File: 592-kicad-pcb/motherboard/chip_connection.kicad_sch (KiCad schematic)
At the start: 28 parts, among them J3 DF40C-40DP-0.4V(51), J4 DF40C-40DP-0.4V(51), J5 Conn_01x16, J6 Conn_01x16, J7 Conn_01x16

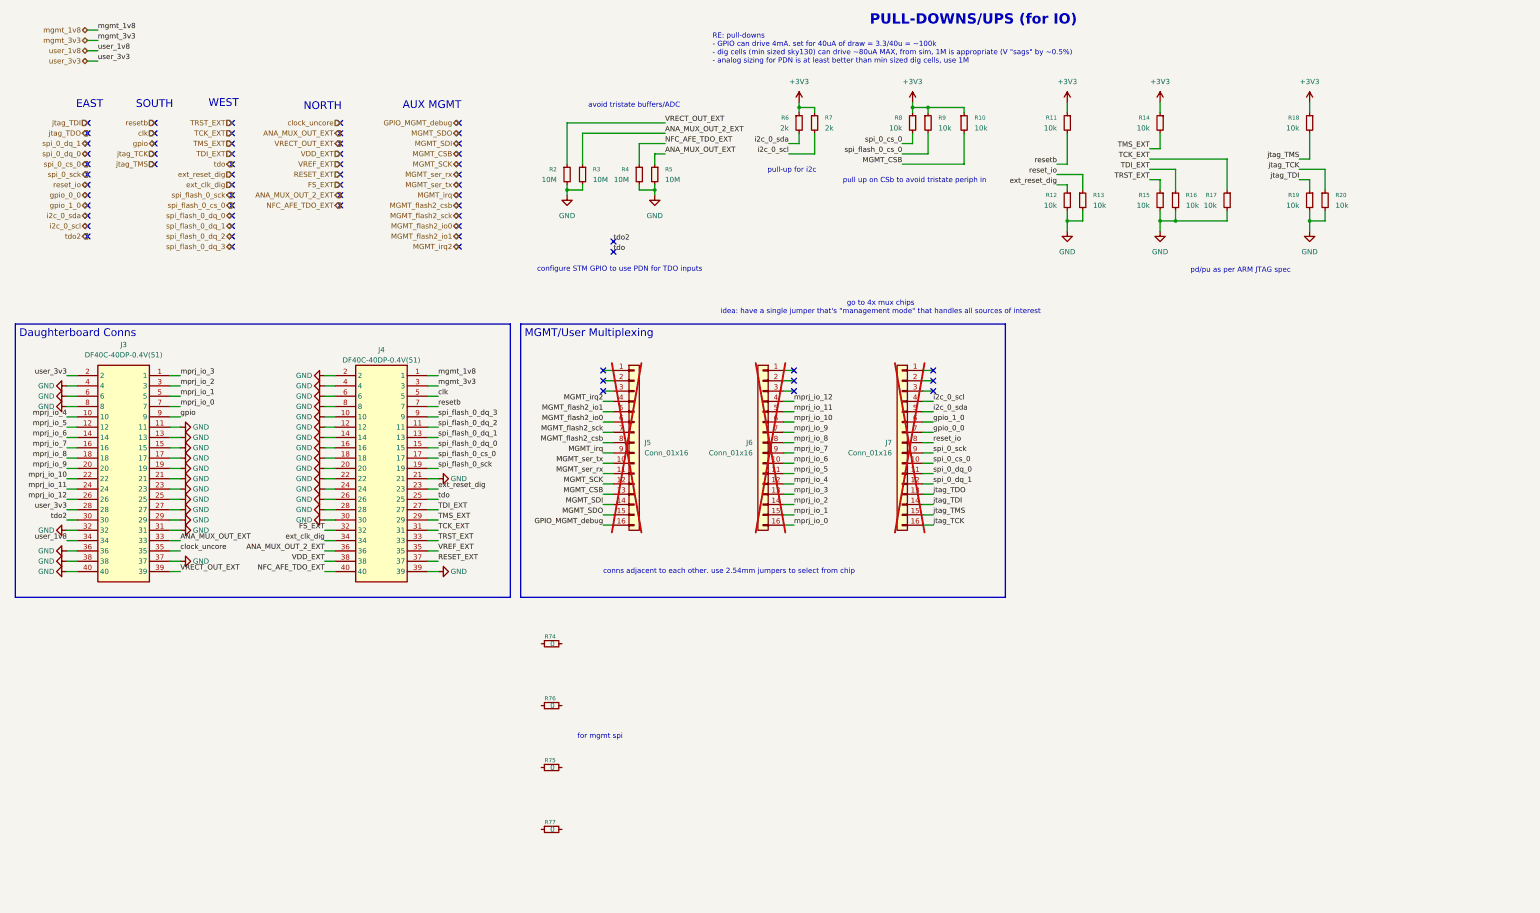
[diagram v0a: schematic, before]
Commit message: finalize termination
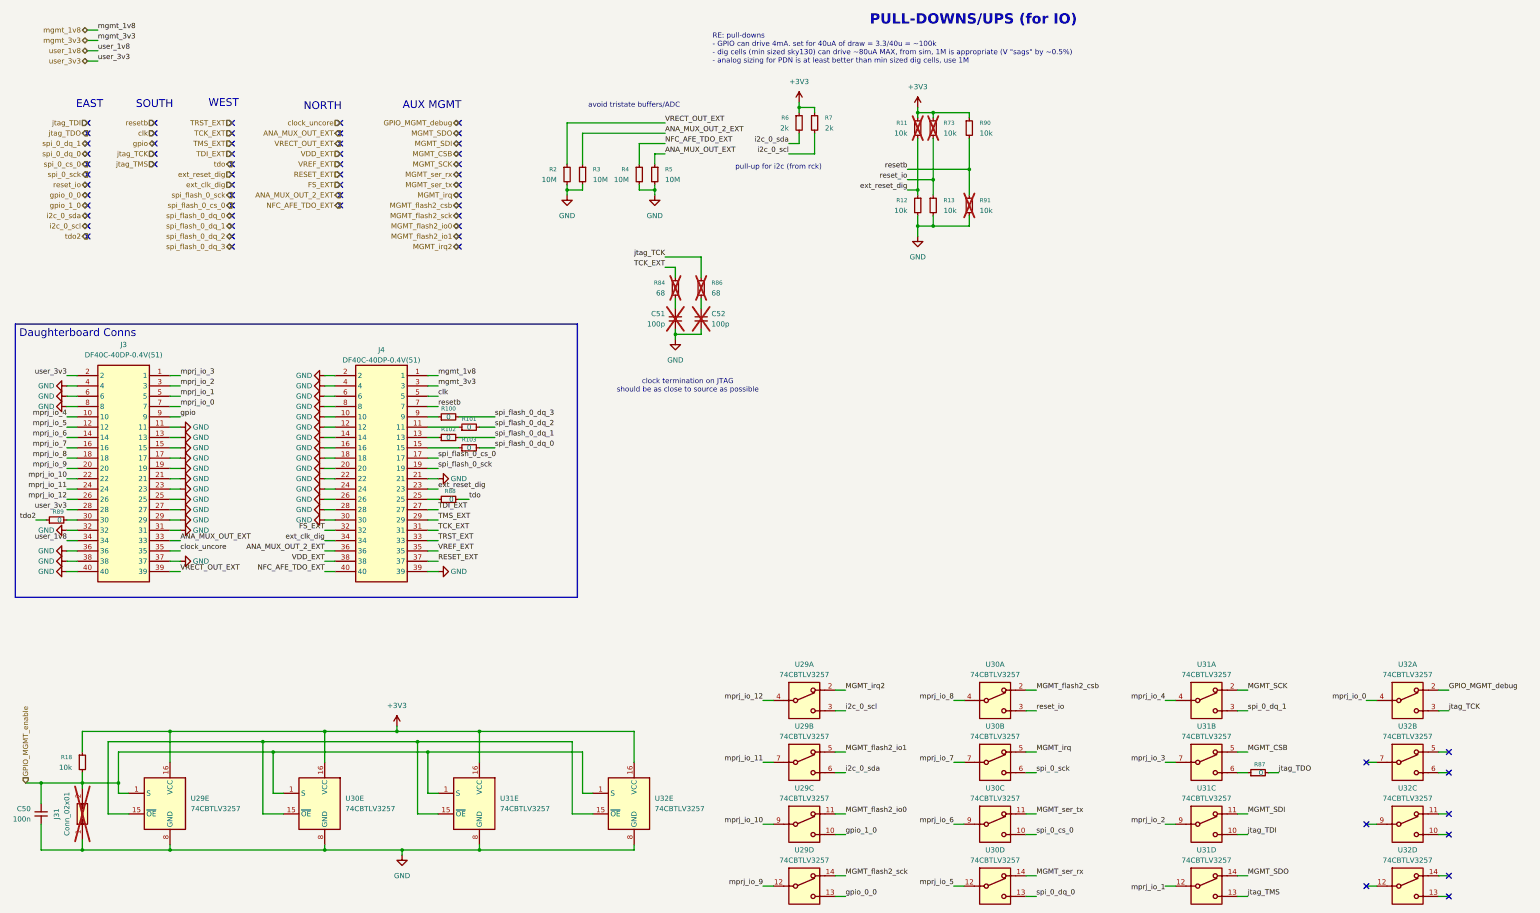
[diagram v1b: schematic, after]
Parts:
- removed J5, J6, J7: Conn_01x16, Connector_PinHeader_2.54mm:PinHeader_1x16_P2.54mm_Vertical, symbol Connector_Generic:Conn_01x16
- removed R10, R14, R15, R16, R17, R19, R20, R8, R9: 10k, Resistor_SMD:R_0603_1608Metric, symbol Device:R_Small
- removed R74, R75, R76, R77: 0, Resistor_SMD:R_0402_1005Metric, symbol Device:R_Small
- added C50: 100n, Capacitor_SMD:C_0402_1005Metric, symbol Device:C_Small
- added C51, C52: 100p, symbol Device:C_Small
- added J31: Conn_02x01, Connector_PinHeader_1.27mm:PinHeader_1x02_P1.27mm_Vertical, symbol Connector_Generic:Conn_02x01
- added R100, R101, R102, R103, R87, R88, R89: 0, symbol Device:R_Small
- added R73, R90, R91: 10k, Resistor_SMD:R_0603_1608Metric, symbol Device:R_Small
- added R84, R86: 68, symbol Device:R_Small
- added U29, U30, U31, U32: 74CBTLV3257, symbol 74xx:74CBTLV3257
- R11: now not fitted
- R18: footprint Resistor_SMD:R_0603_1608Metric -> Resistor_SMD:R_0402_1005Metric; LCSC C25804 -> C25744
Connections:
- net +3V3: now also R73.1, R90.1, U29.16 (VCC), U30.16 (VCC), U31.16 (VCC), U32.16 (VCC)
- net GND: now also C50.2, C51.2, C52.2, J31.1 (Pin_1), R91.2, U29.8 (GND), U30.8 (GND), U31.8 (GND), U32.8 (GND)
- net GPIO_MGMT_debug: now also U32.2
- net MGMT_CSB: now also U31.5
- net MGMT_SCK: now also U31.2
- net MGMT_SDI: now also U31.11
- net MGMT_SDO: now also U31.14
- net MGMT_flash2_csb: now also U30.2
- net MGMT_flash2_io0: now also U29.11
- net MGMT_flash2_io1: now also U29.5
- net MGMT_flash2_sck: now also U29.14
- net MGMT_irq: now also U30.5
- net MGMT_irq2: now also U29.2
- net MGMT_ser_rx: now also U30.14
- net MGMT_ser_tx: now also U30.11
- net TCK_EXT: now also R84.1
- net ext_reset_dig: now also R11.2
- net gpio_0_0: now also U29.13
- net gpio_1_0: now also U29.10
- net i2c_0_scl: now also U29.3
- net i2c_0_sda: now also U29.6
- net jtag_TCK: now also R86.1, U32.3
- net jtag_TDI: now also U31.10
- net jtag_TDO: now also R87.2
- net jtag_TMS: now also U31.13; no longer R18.2
- net mprj_io_0: now also U32.4
- net mprj_io_10: now also U29.9
- net mprj_io_11: now also U29.7
- net mprj_io_12: now also U29.4
- net mprj_io_2: now also U31.9
- net mprj_io_3: now also U31.7
- net mprj_io_4: now also U31.4
- net mprj_io_5: now also U30.12
- net mprj_io_6: now also U30.9
- net mprj_io_7: now also U30.7
- net mprj_io_8: now also U30.4
- net mprj_io_9: now also U29.12
- net reset_io: now also R73.2, U30.3
- net resetb: now also R90.2, R91.1; no longer R11.2
- net spi_0_cs_0: now also U30.10
- net spi_0_dq_0: now also U30.13
- net spi_0_dq_1: now also U31.3
- net spi_0_sck: now also U30.6
- net spi_flash_0_dq_0: now also R103.2; no longer J4.15
- net spi_flash_0_dq_1: now also R102.2; no longer J4.13
- net spi_flash_0_dq_2: now also R101.2; no longer J4.11
- net spi_flash_0_dq_3: now also R100.2; no longer J4.9
- net tdo: now also R88.2; no longer J4.25
- net tdo2: now also R89.1; no longer J3.30
- new net: J4.11, R101.1
- new net: J4.13, R102.1
- new net: J4.15, R103.1
- new net: J4.25, R88.1
- new net: J4.9, R100.1
- new net: C51.1, R84.2
- new net: U29.15 (~{OE}), U30.15 (~{OE}), U31.15 (~{OE}), U32.15 (~{OE})
- new net: R87.1, U31.6
- new net: J3.30, R89.2
- new net: C52.1, R86.2
- new net GPIO_MGMT_enable: C50.1, J31.2 (Pin_2), R18.2, U29.1 (S), U30.1 (S), U31.1 (S), U32.1 (S)
- no-connect marks 63 -> 61
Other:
- note added: "clock termination on JTAG should be as close to source as possible"
- note added: "pull-up for i2c (from rck)"
- note removed: "configure STM GPIO to use PDN for TDO inputs"
- note removed: "conns adjacent to each other. use 2.54mm jumpers to select from chip"
- note removed: "for mgmt spi"
- note removed: "go to 4x mux chips idea: have a single jumper that's "management mode" that handles all sources of interest"
- note removed: "pd/pu as per ARM JTAG spec"
- note removed: "pull up on CSb to avoid tristate periph in"
- note removed: "pull-up for i2c"
- moved on the sheet: R12, R13
